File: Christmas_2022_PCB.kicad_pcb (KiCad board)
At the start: 2 copper layers, 64 x 61 mm, 31 parts, among them J1 USB_A, SW1 SW_Push, SW2 SW_Push, SW3 SW_SPDT, U1 STM32F030K6Tx, U2 AMS1117-3.3

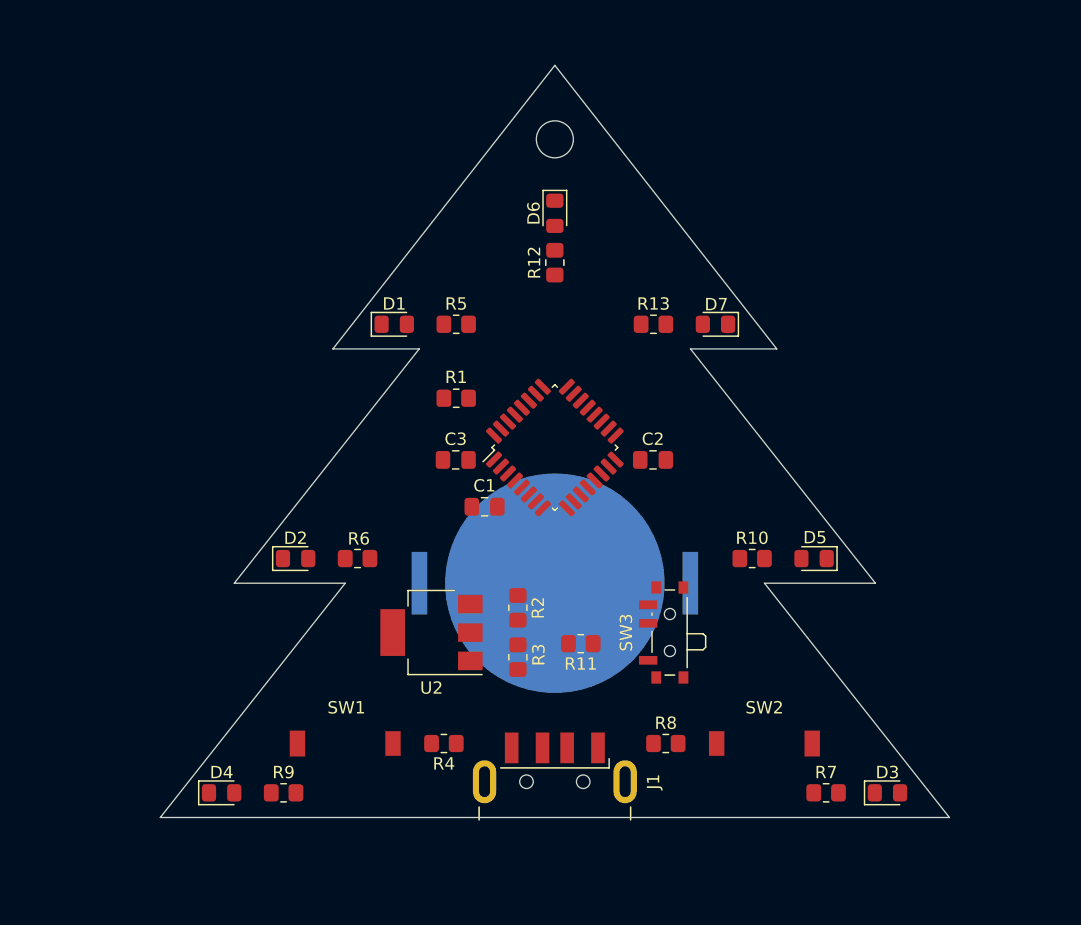
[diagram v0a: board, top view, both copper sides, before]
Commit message: began routing
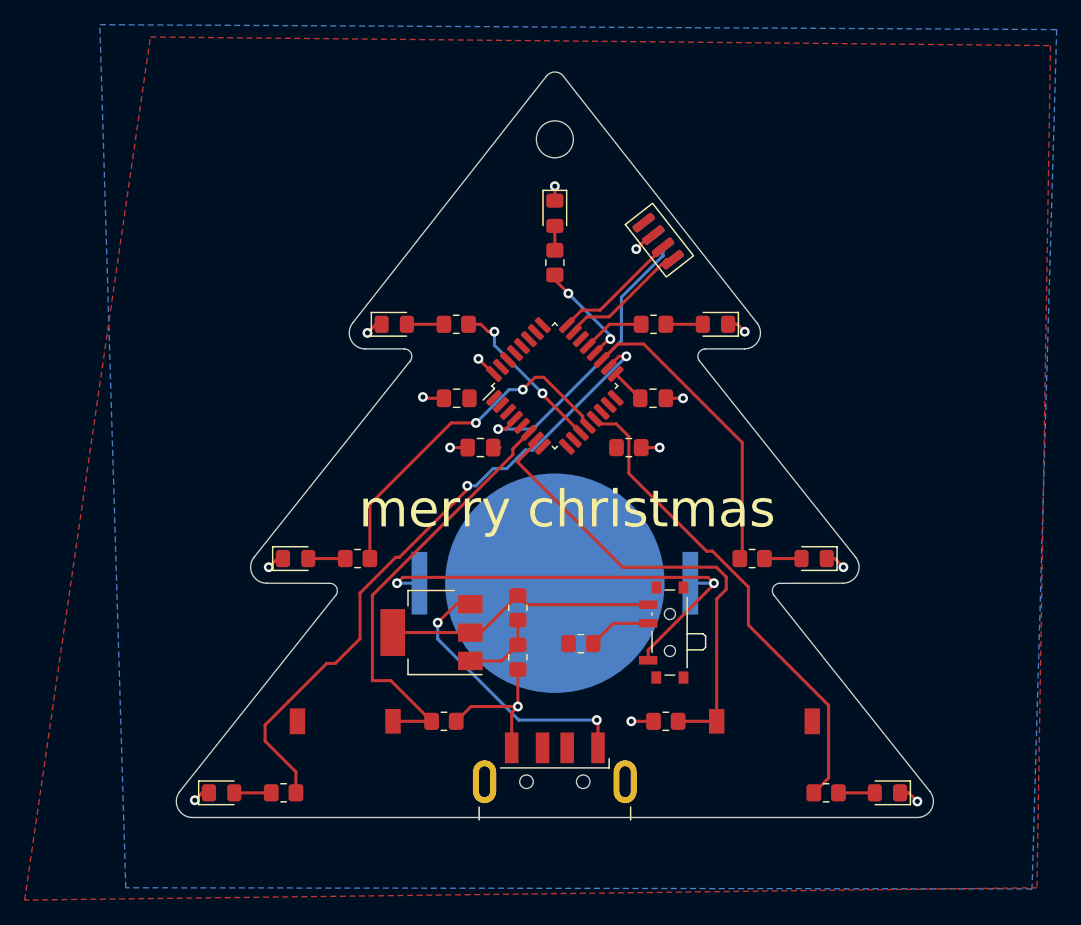
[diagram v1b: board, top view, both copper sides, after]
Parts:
- added J2: SOP8_test_point, Library:sop_8_test_pad, F.Cu at (98.5, 63.2)
- added J3: SOP8_test_point, Library:sop_8_test_pad, B.Cu at (98.5, 63.2)
- moved R1 14.6 mm to (96.0, 80.0), turned to 0 degrees
- moved C3 5.00 mm to (82.0, 76.0), turned to 180 degrees
- moved C2 5.00 mm to (98.0, 76.0)
- moved U1 5.00 mm to (90.0, 75.0)
- moved C1 4.81 mm to (84.0, 80.0)
- moved R4 1.80 mm to (81.0, 102.2)
- moved R8 1.80 mm to (99.0, 102.2)
- moved SW1 1.80 mm to (73.0, 102.2)
- moved SW2 1.80 mm to (107.0, 102.2)
- turned D3 to 180 degrees
- turned R3 to -90 degrees
- turned R5 to 180 degrees
- turned R9 to 180 degrees
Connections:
- U1 pad 4: unconnected-(U1-Pad4) -> /NRST
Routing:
- net /LED4: track 0.00 -> 52.4 mm, vias 0 -> 2
- net /LED3: track 0.00 -> 39.8 mm
- net /BUT_RIGHT: track 0.00 -> 38.3 mm
- net /VBATT: track 0.00 -> 38.3 mm, vias 0 -> 2
- net /BUT_LEFT: track 0.00 -> 34.7 mm
- net GND: track 0.00 -> 33.9 mm, vias 0 -> 15
- net /LED2: track 0.00 -> 28.2 mm, vias 0 -> 2
- net /LED5: track 0.00 -> 24.7 mm
- net /NRST: track 0.00 -> 23.7 mm, vias 0 -> 1
- net Net-(J1-Pad1): track 0.00 -> 22.5 mm, vias 0 -> 2
- net /VREG: track 0.00 -> 22.3 mm
- net /LED1: track 0.00 -> 13.5 mm, vias 0 -> 2
- net /SWDIO: track 0.00 -> 10.5 mm
- net /SWCLK: track 0.00 -> 10.4 mm
- net /LED6: track 0.00 -> 8.80 mm, vias 0 -> 2
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- added copper zone on F.Cu, net +3V3
- added copper zone on B.Cu, net GND
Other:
- board size 64 x 61 mm -> 61.4 x 60.5 mm
- board text added: "merry christmas"
